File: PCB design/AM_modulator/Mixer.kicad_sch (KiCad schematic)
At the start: 8 parts

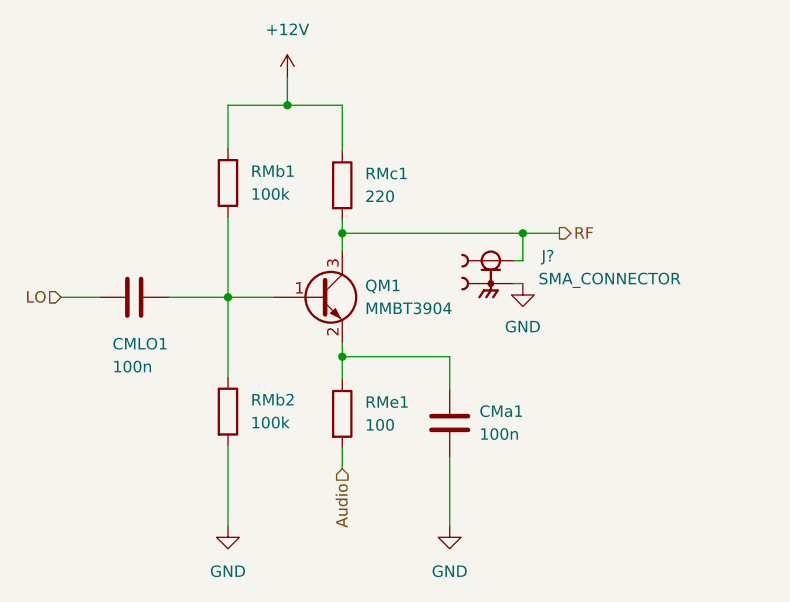
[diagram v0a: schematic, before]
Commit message: PCB 2.0
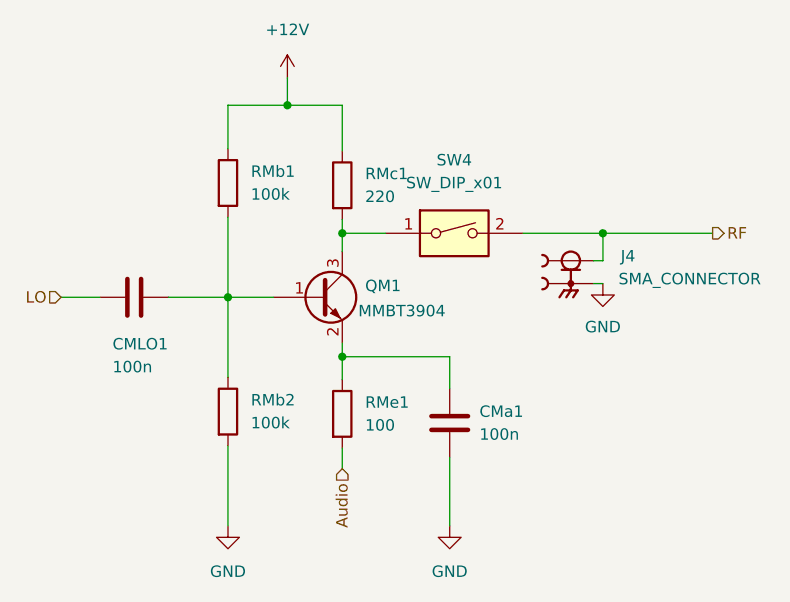
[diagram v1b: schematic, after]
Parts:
- added SW4: SW_DIP_x01, Resistor_SMD:R_0603_1608Metric_Pad0.98x0.95mm_HandSolder, symbol Switch:SW_DIP_x01
- J4: renamed from J?; footprint LPRS_SMA_CONNECTOR -> SMA_T:LPRS_SMA_CONNECTOR
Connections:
- net RF: now also SW4.2; no longer QM1.3 (C), RMc1.2
- new net: QM1.3 (C), RMc1.2, SW4.1
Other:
- moved on the sheet: J4
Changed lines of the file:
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@@
   (junction (at 139.192 81.788) (diameter 0) (color 0 0 0 0)
   )
-  (junction (at 159.258 81.788) (diameter 0) (color 0 0 0 0)
+  (junction (at 168.148 81.788) (diameter 0) (color 0 0 0 0)
   )
   (wire (pts (xy 139.192 105.664) (xy 139.192 107.95))
     (stroke (width 0) (type default) (color 0 0 0 0))
   )
-  (wire (pts (xy 159.258 81.788) (xy 159.258 84.836))
+  (wire (pts (xy 168.148 81.788) (xy 168.148 84.836))
     (stroke (width 0) (type default) (color 0 0 0 0))
   )
@@
   )
   (wire (pts (xy 151.13 106.68) (xy 151.13 114.3))
+    (stroke (width 0) (type default) (color 0 0 0 0))
+  )
+  (wire (pts (xy 168.148 81.788) (xy 180.34 81.788))
     (stroke (width 0) (type default) (color 0 0 0 0))
   )
@@
     (stroke (width 0) (type default) (color 0 0 0 0))
   )
-  (wire (pts (xy 158.242 87.376) (xy 159.258 87.376))
+  (wire (pts (xy 167.132 87.376) (xy 168.148 87.376))
     (stroke (width 0) (type default) (color 0 0 0 0))
   )
@@
   )
   (wire (pts (xy 126.492 88.9) (xy 126.492 97.79))
-    (stroke (width 0) (type default) (color 0 0 0 0))
-  )
-  (wire (pts (xy 159.258 81.788) (xy 163.322 81.788))
     (stroke (width 0) (type default) (color 0 0 0 0))
   )
@@
     (stroke (width 0) (type default) (color 0 0 0 0))
   )
+  (wire (pts (xy 159.258 81.788) (xy 168.148 81.788))
+    (stroke (width 0) (type default) (color 0 0 0 0))
+  )
   (wire (pts (xy 133.096 64.516) (xy 133.096 67.564))
     (stroke (width 0) (type default) (color 0 0 0 0))
   )
-  (wire (pts (xy 139.192 81.788) (xy 159.258 81.788))
+  (wire (pts (xy 139.192 81.788) (xy 144.018 81.788))
     (stroke (width 0) (type default) (color 0 0 0 0))
   )
-  (wire (pts (xy 159.258 84.836) (xy 158.242 84.836))
+  (wire (pts (xy 168.148 84.836) (xy 167.132 84.836))
     (stroke (width 0) (type default) (color 0 0 0 0))
   )
@@
     (stroke (width 0) (type default) (color 0 0 0 0))
   )
-  (hierarchical_label "RF" (shape output) (at 163.322 81.788 0)
+  (hierarchical_label "RF" (shape output) (at 180.34 81.788 0)
     (effects (font (size 1.27 1.27)) (justify left))
   )
@@
     (effects (font (size 1.27 1.27)) (justify right))
   )
-  (symbol (lib_id "power:GND") (at 159.258 87.376 0) (unit 1)
+  (symbol (lib_id "power:GND") (at 168.148 87.376 0) (unit 1)
     (in_bom yes) (on_board yes) (fields_autoplaced)
-    (property "Reference" "#PWR0117" (id 0) (at 159.258 93.726 0)
+    (property "Reference" "#PWR0117" (id 0) (at 168.148 93.726 0)
       (effects (font (size 1.27 1.27)) hide)
     )
-    (property "Value" "GND" (id 1) (at 159.258 92.202 0))
-    (property "Footprint" "" (id 2) (at 159.258 87.376 0)
+    (property "Value" "GND" (id 1) (at 168.148 92.202 0))
+    (property "Footprint" "" (id 2) (at 168.148 87.376 0)
       (effects (font (size 1.27 1.27)) hide)
     )
-    (property "Datasheet" "" (id 3) (at 159.258 87.376 0)
+    (property "Datasheet" "" (id 3) (at 168.148 87.376 0)
       (effects (font (size 1.27 1.27)) hide)
     )
@@
     (pin "2")
   )
-  (symbol (lib_id "SMA_T:SMA_CONNECTOR") (at 155.702 84.836 0) (unit 1)
+  (symbol (lib_id "Switch:SW_DIP_x01") (at 151.638 81.788 0) (unit 1)
+    (in_bom yes) (on_board yes) (fields_autoplaced)
+    (property "Reference" "SW4" (id 0) (at 151.638 73.66 0))
+    (property "Value" "SW_DIP_x01" (id 1) (at 151.638 76.2 0))
+    (property "Footprint" "Resistor_SMD:R_0603_1608Metric_Pad0.98x0.95mm_HandSolder" (id 2) (at 151.638 81.788 0)
+      (effects (font (size 1.27 1.27)) hide)
+    )
+    (property "Datasheet" "~" (id 3) (at 151.638 81.788 0)
+      (effects (font (size 1.27 1.27)) hide)
+    )
+    (pin "1")
+    (pin "2")
+  )
+  (symbol (lib_id "SMA_T:SMA_CONNECTOR") (at 164.592 84.836 0) (unit 1)
     (in_bom yes) (on_board yes)
-    (property "Reference" "J?" (id 0) (at 162.052 84.328 0))
-    (property "Value" "SMA_CONNECTOR" (id 1) (at 168.91 86.868 0))
-    (property "Footprint" "LPRS_SMA_CONNECTOR" (id 2) (at 155.702 84.836 0)
+    (property "Reference" "J4" (id 0) (at 170.942 84.328 0))
+    (property "Value" "SMA_CONNECTOR" (id 1) (at 177.8 86.868 0))
+    (property "Footprint" "SMA_T:LPRS_SMA_CONNECTOR" (id 2) (at 164.592 84.836 0)
       (effects (font (size 1.27 1.27)) (justify left bottom) hide)
     )
-    (property "Datasheet" "" (id 3) (at 155.702 84.836 0)
+    (property "Datasheet" "" (id 3) (at 164.592 84.836 0)
       (effects (font (size 1.27 1.27)) (justify left bottom) hide)
     )
-    (property "MANUFACTURER" "LPRS" (id 4) (at 155.702 84.836 0)
+    (property "MANUFACTURER" "LPRS" (id 4) (at 164.592 84.836 0)
       (effects (font (size 1.27 1.27)) (justify left bottom) hide)
     )
-    (property "MAXIMUM_PACKAGE_HEIGHT" "8.3 mm" (id 5) (at 155.702 84.836 0)
+    (property "MAXIMUM_PACKAGE_HEIGHT" "8.3 mm" (id 5) (at 164.592 84.836 0)
       (effects (font (size 1.27 1.27)) (justify left bottom) hide)
     )
-    (property "STANDARD" "Manufacturer Recommendations" (id 6) (at 155.702 84.836 0)
+    (property "STANDARD" "Manufacturer Recommendations" (id 6) (at 164.592 84.836 0)
       (effects (font (size 1.27 1.27)) (justify left bottom) hide)
     )
-    (property "PARTREV" "1.3" (id 7) (at 155.702 84.836 0)
+    (property "PARTREV" "1.3" (id 7) (at 164.592 84.836 0)
       (effects (font (size 1.27 1.27)) (justify left bottom) hide)
     )
@@
   )
   (symbol (lib_id "Device:Q_NPN_BEC") (at 136.652 88.9 0) (unit 1)
-    (in_bom yes) (on_board yes) (fields_autoplaced)
+    (in_bom yes) (on_board yes)
     (property "Reference" "QM1" (id 0) (at 141.732 87.6299 0)
       (effects (font (size 1.27 1.27)) (justify left))
     )
-    (property "Value" "MMBT3904" (id 1) (at 141.732 90.1699 0)
+    (property "Value" "MMBT3904" (id 1) (at 140.97 90.424 0)
       (effects (font (size 1.27 1.27)) (justify left))
     )
